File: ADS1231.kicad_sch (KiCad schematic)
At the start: 1 part, among them U13 ADS1231ID

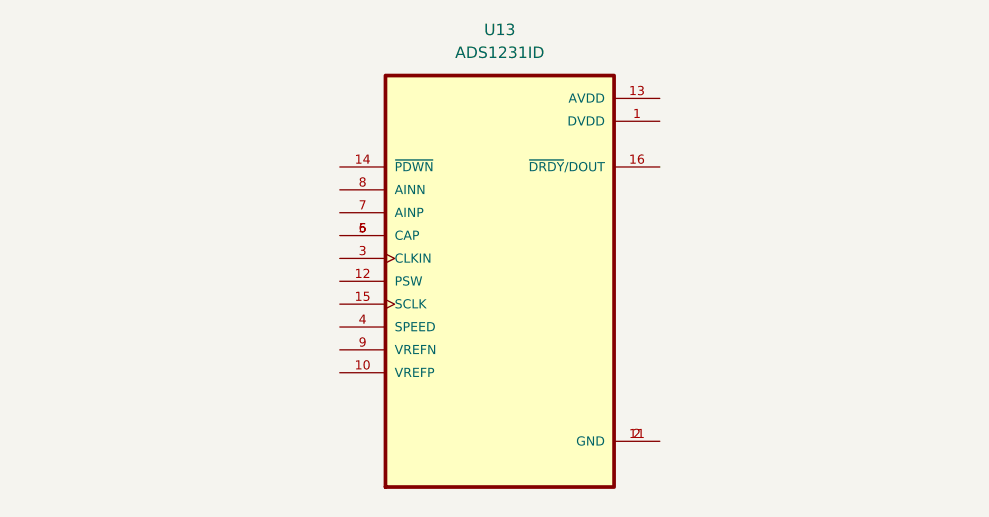
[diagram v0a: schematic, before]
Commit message: Added Load Cell IC and Circuitry, fixed wacked out symbol
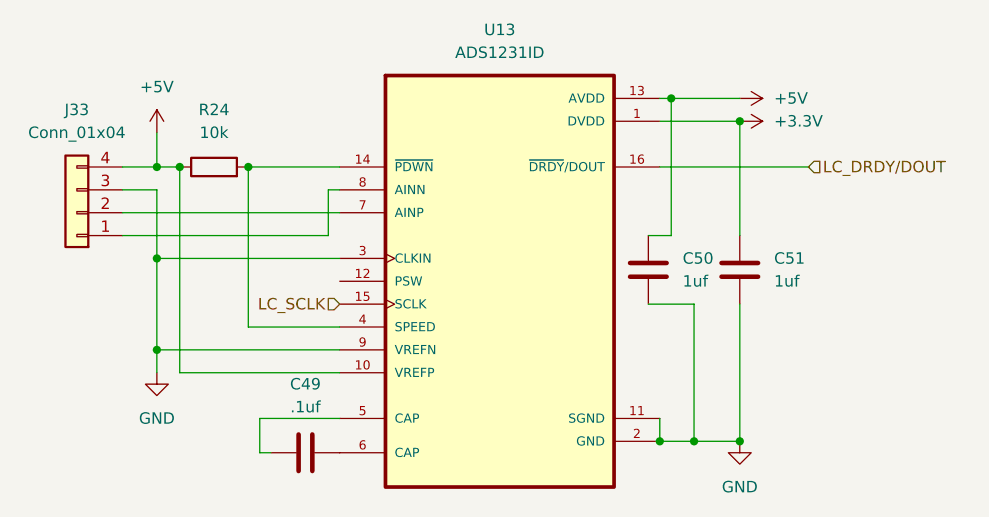
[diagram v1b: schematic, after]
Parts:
- added C49: .1uf, Capacitor_SMD:C_0402_1005Metric, symbol Device:C
- added C50, C51: 1uf, Capacitor_SMD:C_0402_1005Metric, symbol Device:C
- added J33: Conn_01x04, symbol Connector_Generic:Conn_01x04
- added R24: 10k, Resistor_SMD:R_0402_1005Metric, symbol Device:R
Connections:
- net +3.3V: now reaches U13.1 (DVDD)
- net +3.3V: now also C51.2
- net +5V: now reaches U13.10 (VREFP)
- net +5V: now also U13.13 (AVDD), C50.1, J33.4 (Pin_4), R24.1
- net GND: now reaches U13.11 (SGND), U13.2 (GND)
- net GND: now also U13.3 (CLKIN), U13.9 (VREFN), C50.2, C51.1, J33.3 (Pin_3)
- net at U13.14 (~{PDWN}): now also U13.4 (SPEED), R24.2
- net LC_SCLK: now reaches U13.15 (SCLK)
- net LC_DRDY/DOUT: now reaches U13.16 (~{DRDY}/DOUT)
- net at U13.5 (CAP): now also C49.2; no longer U13.6 (CAP)
- net at U13.7 (AINP): now also J33.2 (Pin_2)
- net at U13.8 (AINN): now also J33.1 (Pin_1)
- new net: C49.1, U13.6 (CAP)
